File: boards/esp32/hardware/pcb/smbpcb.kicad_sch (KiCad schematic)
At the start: 61 parts, among them IC1 MiCS-6814, J1 USB_B_Micro, J2 PMS7003, Q1 SUD08P06-155L, SW1 RESET, SW2 RESET, U1 MCP73831-2-OT, U2 SGM6603-5.0YN6G_TR, U3 ESP32-WROOM-32, U4 SSD1306, U5 BME680, U6 MH-Z19B, U7 AMS1117-3.3

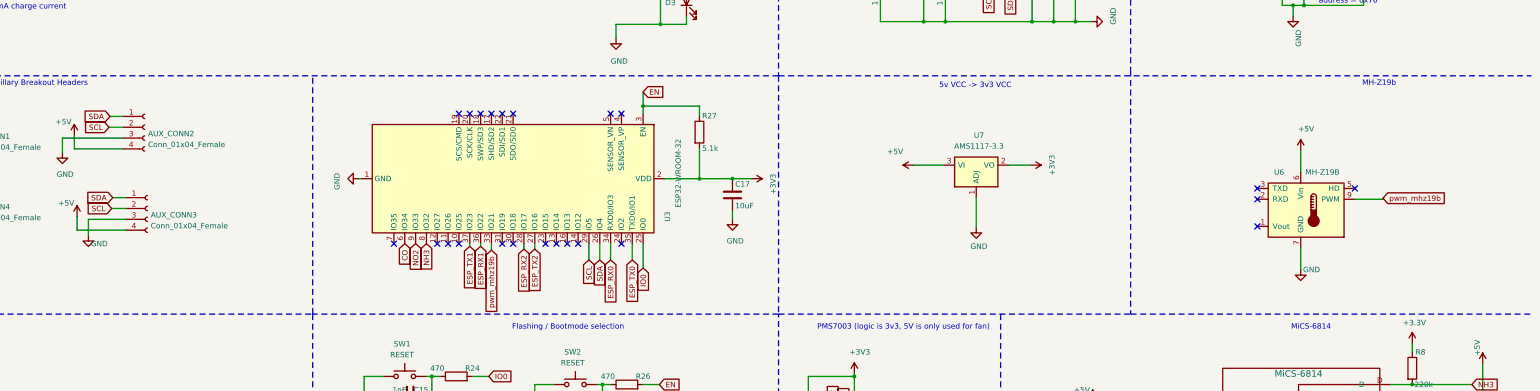
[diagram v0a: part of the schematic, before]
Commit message: moving stuff
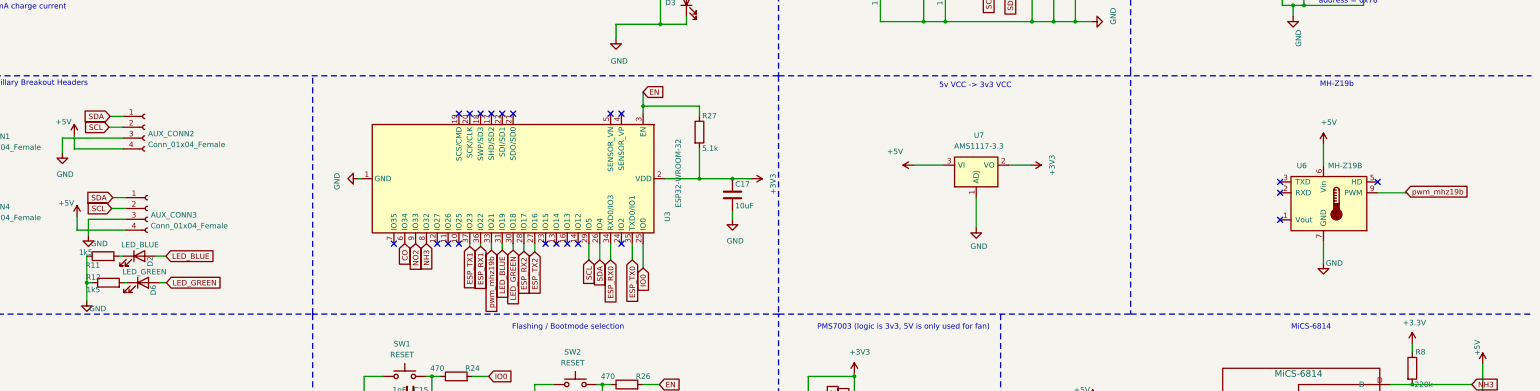
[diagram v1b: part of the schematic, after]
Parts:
- added D2: LED_BLUE, Capacitor_SMD:C_0805_2012Metric, symbol Device:LED
- added D6: LED_GREEN, Capacitor_SMD:C_0805_2012Metric, symbol Device:LED
- added R11, R12: 1k5, symbol Device:R
- SW1, SW2: mfr_part_num ST-1102W-4.3 -> (none)
- U4: footprint mics:SSD1306_OLED-0.91-128x32 -> stuff:SSD1306_OLED-0.91-128x32
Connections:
- net GND: now also R11.1, R12.1
- net LED_GREEN: now reaches U3.30 (IO18)
- net LED_GREEN: now also D6.2 (A)
- net LED_BLUE: now reaches U3.31 (IO19)
- net LED_BLUE: now also D2.2 (A)
- new net: D2.1 (K), R11.2
- new net: D6.1 (K), R12.2
- no-connect marks 26 -> 24
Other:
- moved on the sheet: U6
